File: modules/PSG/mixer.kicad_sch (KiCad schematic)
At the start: 28 parts, among them J2 MonoJack, P1 10kΩ, U2 LM386N-4, U3 TL072

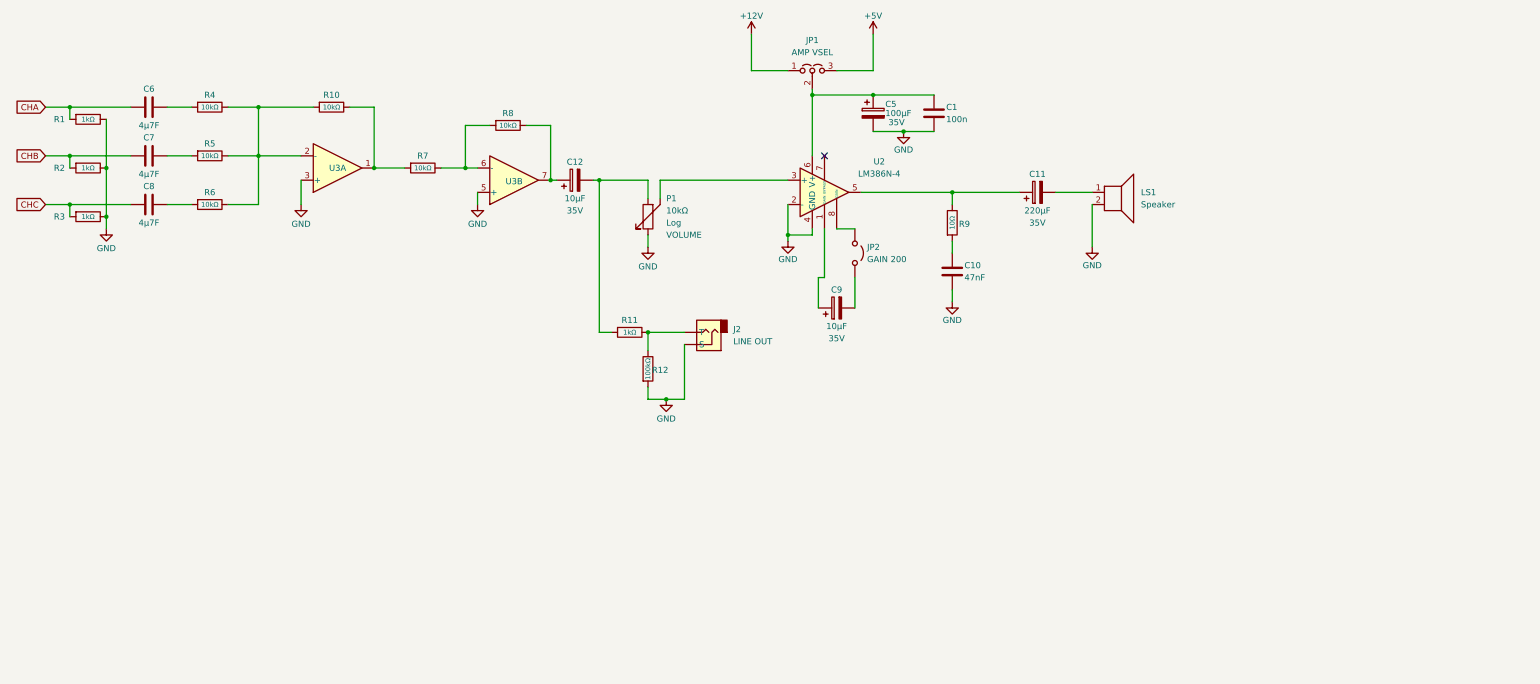
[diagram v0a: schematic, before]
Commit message: sync
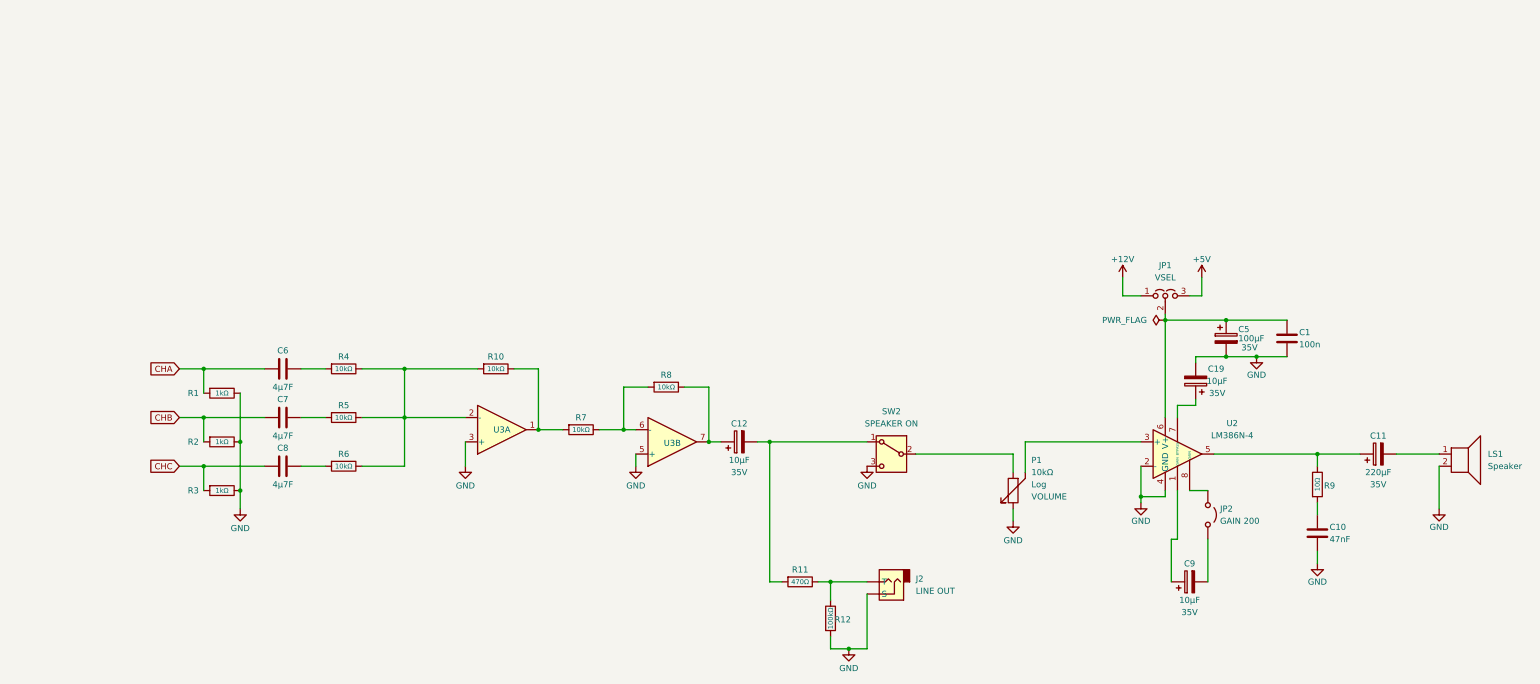
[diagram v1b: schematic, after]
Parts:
- added C19: 10µF, IMNOTWOPR:CP_Radial_Tantal_P100mil, symbol IMNOTWOPR:C_Polarized
- added SW2: SPEAKER ON, IMNOTWOPR:PanelConnector_1x03, symbol IMNOTWOPR:SW_SPDT
- JP1: value AMP VSEL -> VSEL
- R11: value 1kΩ -> 470Ω
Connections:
- net GND: now also C19.2, SW2.3 (C)
- net at U2.7 (BYPASS): now also C19.1
- net at C12.2, R11.2: now also SW2.1 (A); no longer P1.3
- new net: P1.3, SW2.2 (B)
- no-connect marks 1 -> 0
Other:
- company: (none) -> THE HOUSE OF GALAHAD
- title: (none) -> PSG
- moved on the sheet: C1, C10, C11, C12, C5, C6, C7, C8, C9, J2, JP1, JP2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
